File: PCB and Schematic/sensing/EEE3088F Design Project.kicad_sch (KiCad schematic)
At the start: 28 parts, among them J1 Conn_02x14_Odd_Even, Q1 2N3904, Q2 2N3904, Q3 2N3904

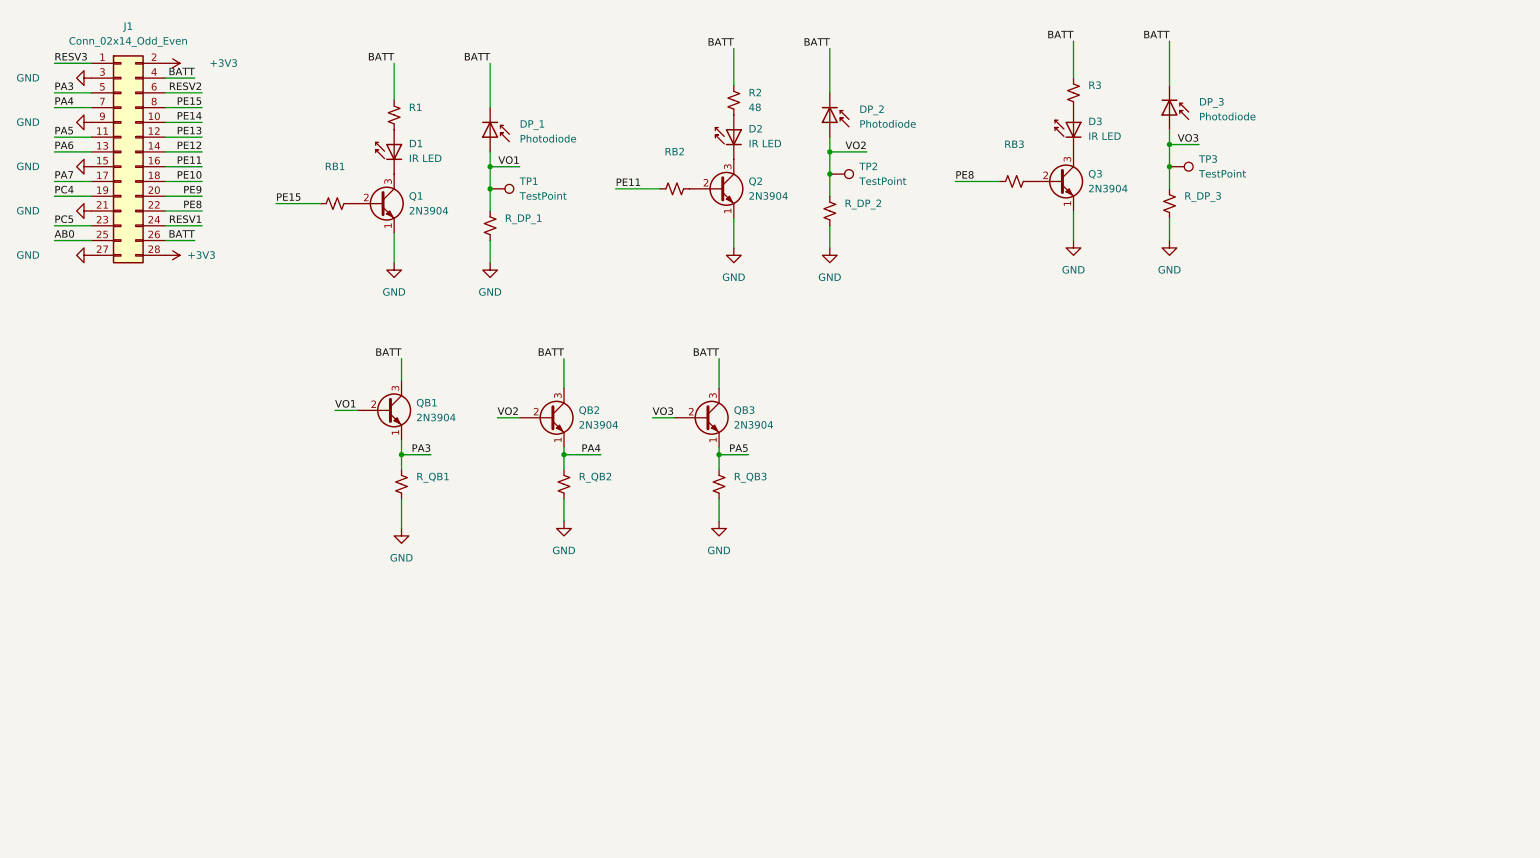
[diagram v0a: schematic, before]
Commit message: Add files via upload
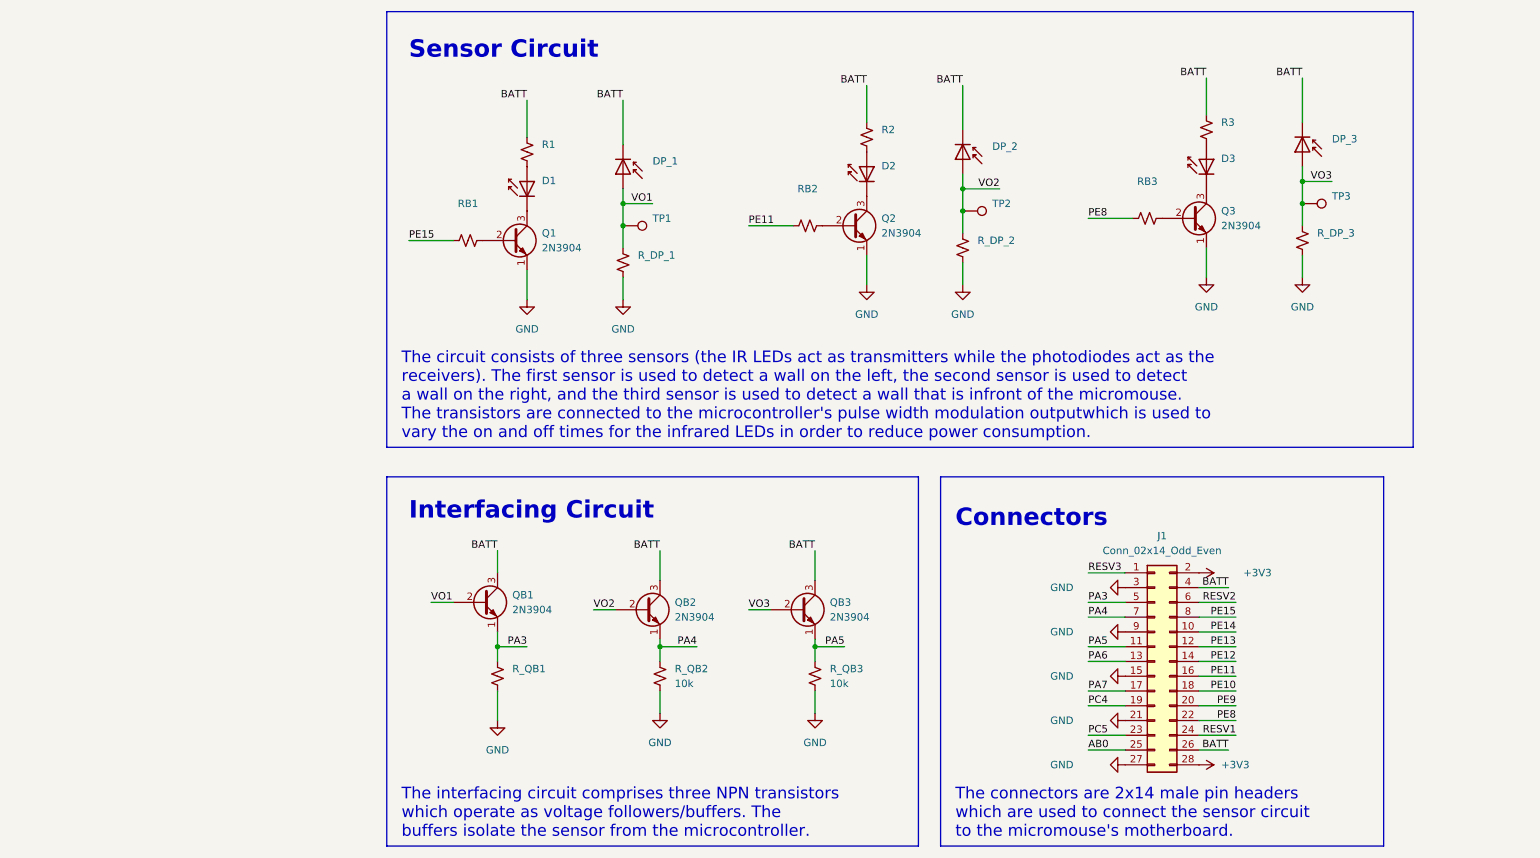
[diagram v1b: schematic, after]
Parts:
- D1, D2, D3: value IR LED -> (none); footprint LED_THT:LED_D5.0mm_Horizontal_O6.35mm_Z3.0mm -> (none)
- DP_1, DP_2, DP_3: value Photodiode -> (none); footprint LED_THT:LED_D3.0mm_Horizontal_O6.35mm_Z2.0mm -> (none); LCSC C264280 -> C2900211
- R1, R3: LCSC (none) -> C2896827
- R2: value 48 -> (none); footprint Resistor_SMD:R_0201_0603Metric -> (none); LCSC (none) -> C2896827
- RB1, RB2, RB3: LCSC (none) -> C120072
- R_DP_1, R_DP_2, R_DP_3: LCSC (none) -> C2894608
- R_QB1: LCSC (none) -> C120262
- R_QB2, R_QB3: value (none) -> 10k; footprint (none) -> Resistor_THT:R_Axial_DIN0204_L3.6mm_D1.6mm_P1.90mm_Vertical; LCSC (none) -> C120262
- TP1, TP2, TP3: value TestPoint -> (none)
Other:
- note added: "Connectors"
- note added: "Interfacing Circuit"
- note added: "Sensor Circuit"
- note added: "The circuit consists of three sensors (the IR LEDs act as transmitters while the photodiodes act as the receivers). The first sensor is used to detect a wall on the left, the second sensor is used to detect a wall on the right, and the third sensor is used to detect a wall that is infront of the micromouse. The transistors are connected to the microcontroller's pulse width modulation outputwhich 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"
- note added: "The connectors are 2x14 male pin headers which are used to connect the sensor circuit to the micromouse's motherboard."
- note added: "The interfacing circuit comprises three NPN transistors which operate as voltage followers/buffers. The buffers isolate the sensor from the microcontroller."
- title: (none) -> EEE3088 Design Project (Micromouse Sensing Module)
- moved on the sheet: D1, D2, D3, DP_1, DP_2, DP_3, J1, Q1, Q2, Q3, QB1, QB2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
